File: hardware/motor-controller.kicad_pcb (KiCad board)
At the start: 2 copper layers, 71.2 x 43 mm, 55 parts, among them P1 VTEST, P101 BATTERY, P102 SWD, P103 EDISON-BULB-E10, P104 FTDI-PLUG, P2 P01, P201 P06-MOTOR, P202 P06-MOTOR, P3 P01, P4 P01, U101 STM32F030K6T6, U102 ST-LIS3MDL, U201 IRLML2803TRPBF, U202 IRLML2803TRPBF, U203 7408, U204 MC33926, U205 MC33926, U206 74AHC541D

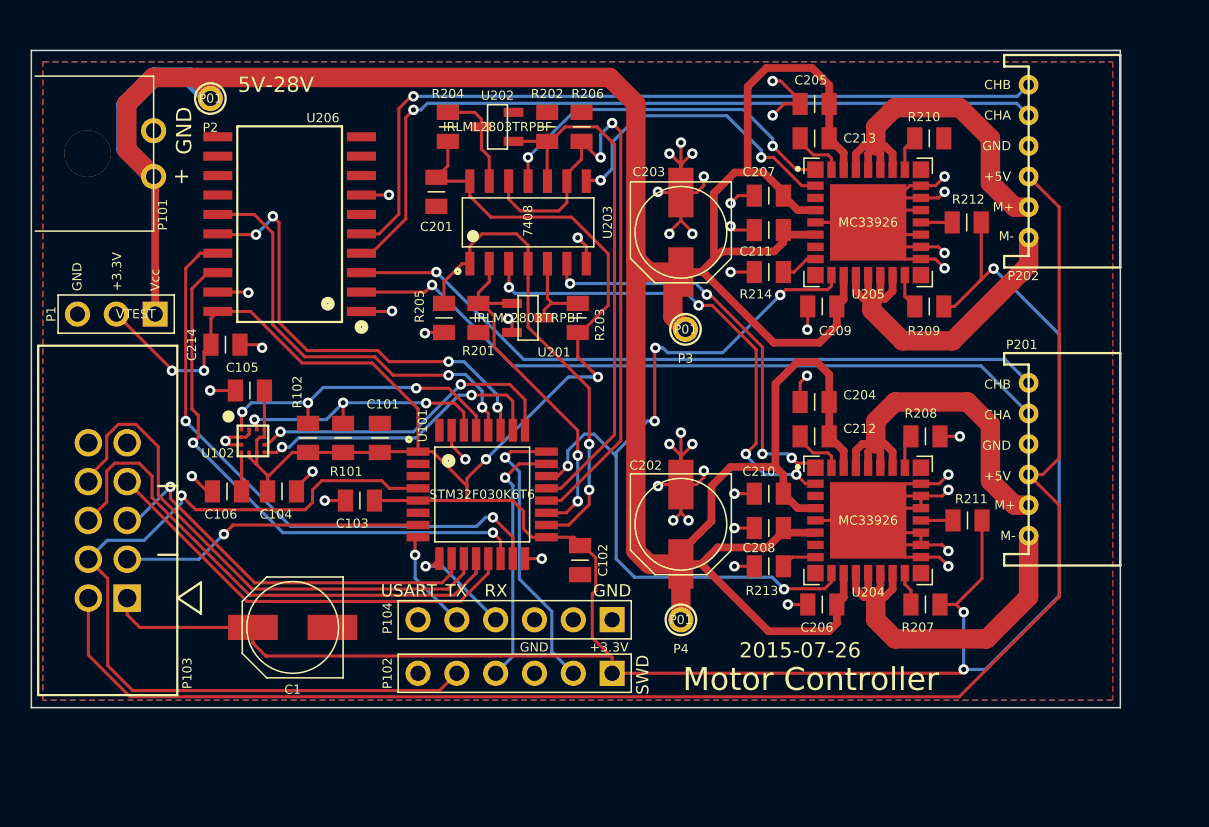
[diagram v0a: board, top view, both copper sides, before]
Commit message: rework layout
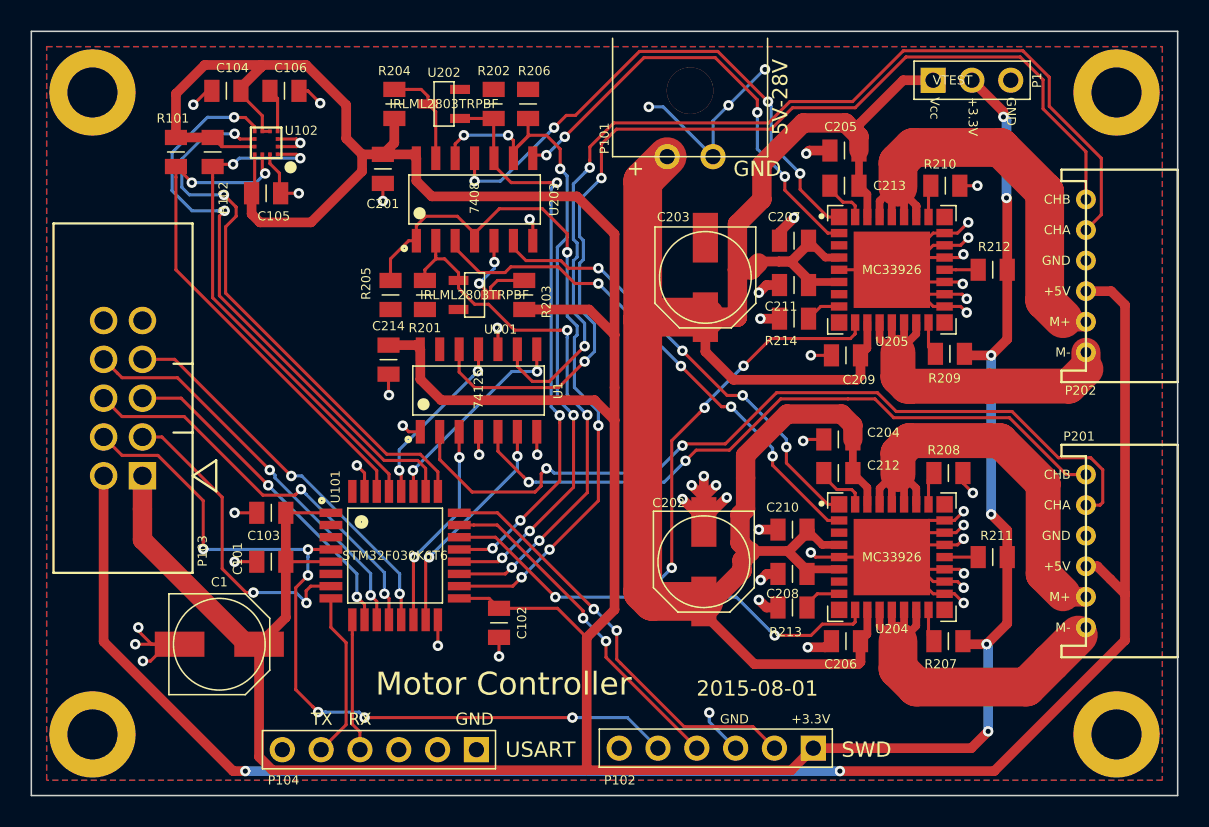
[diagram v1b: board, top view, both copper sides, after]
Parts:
- removed P2, P3, P4: P01, kicadlib:HDRV1W66P254_1X1_254X249X838P-ROUND
- removed U206: 74AHC541D, kicadlib:SOIC127P1032X265-20N
- added M1: Mounting Hole, kicadlib:MTGNP565H328Z565P, F.Cu at (117.0, 146.0)
- added M2: Mounting Hole, kicadlib:MTGNP565H328Z565P, F.Cu at (184.0, 146.0)
- added M3: Mounting Hole, kicadlib:MTGNP565H328Z565P, F.Cu at (184.0, 104.0)
- added M4: Mounting Hole, kicadlib:MTGNP565H328Z565P, F.Cu at (117.0, 104.0)
- added U1: 74125, kicadlib:SOIC127P600X175-14N, F.Cu at (142.3, 123.5)
- moved P1 53.1 mm to (172.0, 103.2), turned to 0 degrees
- moved P101 33.6 mm to (154.6, 108.2), turned to 0 degrees
- moved C106 26.5 mm to (129.6, 103.9), turned to 0 degrees
- moved C104 26.5 mm to (125.8, 103.9), turned to 180 degrees
- moved R101 21.7 mm to (122.5, 107.9), turned to 270 degrees
- moved R102 19.7 mm to (124.9, 107.9), turned to 270 degrees
- moved U102 19.5 mm to (128.4, 107.3), turned to 180 degrees
- moved P102 14.0 mm to (164.2, 146.9)
- moved C105 12.9 mm to (128.4, 110.6), turned to 0 degrees
- moved P104 12.3 mm to (142.1, 147.0)
- moved C101 10.8 mm to (128.7, 134.7), turned to 180 degrees
- moved C214 10.7 mm to (136.4, 121.5), turned to 270 degrees
- moved P202 8.39 mm to (182.0, 116.0)
- moved P103 8.06 mm to (119.0, 124.0)
- moved P201 7.08 mm to (182.0, 134.0)
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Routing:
- net Vcc: track 219.0 -> 154.5 mm
- net +3.3V: track 227.5 -> 271.7 mm, vias 7 -> 6
- net /drivers/MOTORLCHB: track 39.1 -> 14.8 mm
- net /drivers/MOTORLCHA: track 36.5 -> 13.6 mm
- net /COMPASSINT: track 19.9 -> 38.8 mm
- net /I2CSDA: track 17.6 -> 34.6 mm, vias 3 -> 2
- net /drivers/MOTORRCHB: track 28.4 -> 11.5 mm
- net /COMPASSDRDY: track 21.1 -> 37.5 mm
- net /drivers/MOTORRCHA: track 29.9 -> 13.7 mm, vias 4 -> 2
- net /drivers/MOTORLPWM: track 31.2 -> 46.9 mm, vias 2 -> 4
- net /drivers/MOTORROUTCHB: track 51.7 -> 67.4 mm, vias 1 -> 2
- net /drivers/MOTORROUTCHA: track 51.9 -> 66.6 mm, vias 1 -> 2
- net /I2CSCL: track 20.2 -> 33.6 mm, vias 3 -> 2
- net /drivers/MOTORLDIR: track 23.2 -> 35.8 mm, vias 2 -> 4
- net Net-(U203-Pad11): track 23.6 -> 35.5 mm, vias 2 -> 4
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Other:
- board size 71.2 x 43 mm -> 75 x 50 mm
- board text added: "2015-08-01"
- board text removed: "2015-07-26"
